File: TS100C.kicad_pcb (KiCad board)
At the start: 4 copper layers, 84 x 10 mm, 52 parts, among them J1 USB_C, J2 OLED_64x32, J3 A, J4 B, J5 DNP, P1 TC2030-CTX, Q1 SS8050, Q2 DMP3017SFG, SW1 key1, SW2 key2, U1 USBLC6-4SC6, U2 AP2204R-3.3, U3 FUSB302BMPX, U4 STM32F072C8Ux, U5 OPA340NA, U6 MCP9700AT-ETT

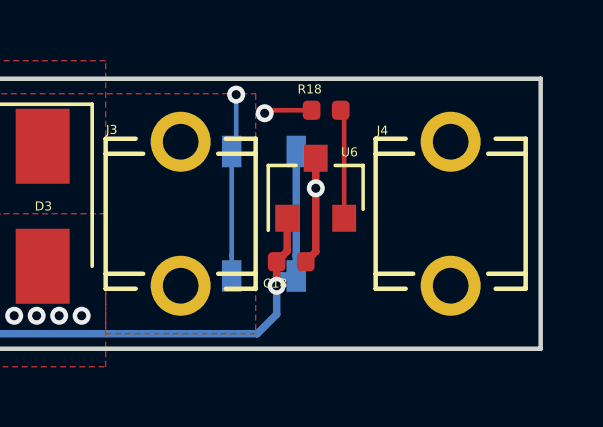
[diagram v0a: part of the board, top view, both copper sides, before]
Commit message: update PCB
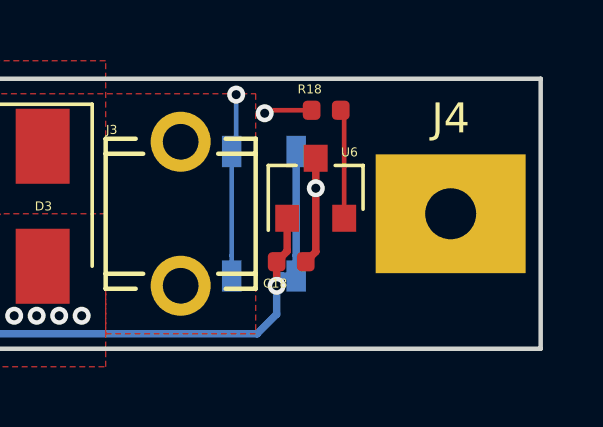
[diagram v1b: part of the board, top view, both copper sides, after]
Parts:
- J4: footprint otter:Keystone_3621 -> otter:3622TR
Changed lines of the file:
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@@
     (add_net nRST)
+  )
+  (module otter:3622TR (layer F.Cu)
+    (at 161 85)
+    (fp_text reference J4 (at 0 -3.175) (layer F.SilkS)
+      (effects (font (size 1 1) (thickness 0.15)))
+    )
+    (fp_text value B (at 0 -5.08) (layer F.Fab)
+      (effects (font (size 1 1) (thickness 0.15)))
+    )
+    (pad 1 thru_hole rect (at 0 0) (size 5 3.96) (drill 1.7) (layers *.Cu *.Mask)
+      (net 1 GND))
   )
   (module Capacitor_SMD:C_0402_1005Metric (layer F.Cu)
@@
     )
   )
-  (module otter:Keystone_3621 (layer F.Cu)
-    (at 161 85)
-    (fp_text reference J4 (at -2.275 -2.775) (layer F.SilkS)
-      (effects (font (size 0.3 0.3) (thickness 0.05)))
-    )
-    (fp_text value B (at 0 -4.5) (layer F.Fab)
-      (effects (font (size 1 1) (thickness 0.15)))
-    )
-    (fp_line (start 1.25 -2) (end 2.5 -2) (layer F.SilkS) (width 0.15))
-    (fp_line (start -2.5 -2) (end -1.25 -2) (layer F.SilkS) (width 0.15))
-    (fp_line (start -1.25 2) (end -2.5 2) (layer F.SilkS) (width 0.15))
-    (fp_line (start 1.25 2) (end 2.5 2) (layer F.SilkS) (width 0.15))
-    (fp_line (start 1.5 -2.5) (end 2.5 -2.5) (layer F.SilkS) (width 0.15))
-    (fp_line (start 2.5 2.5) (end 1.5 2.5) (layer F.SilkS) (width 0.15))
-    (fp_line (start -1.5 -2.5) (end -2.5 -2.5) (layer F.SilkS) (width 0.15))
-    (fp_line (start 2.5 2.5) (end 2.5 -2.5) (layer F.SilkS) (width 0.15))
-    (fp_line (start -2.5 2.5) (end -1.5 2.5) (layer F.SilkS) (width 0.15))
-    (fp_line (start -2.5 -2.5) (end -2.5 2.5) (layer F.SilkS) (width 0.15))
-    (pad 1 thru_hole circle (at 0 2.4) (size 2 2) (drill 1.19) (layers *.Cu *.Mask)
-      (net 1 GND))
-    (pad 1 thru_hole circle (at 0 -2.4) (size 2 2) (drill 1.19) (layers *.Cu *.Mask)
-      (net 1 GND))
-    (model /home/janhenrik/Downloads/keystone-PN3621.STEP
-      (offset (xyz 0 0 0.2))
-      (scale (xyz 1 1 1))
-      (rotate (xyz -90 0 90))
-    )
-  )
